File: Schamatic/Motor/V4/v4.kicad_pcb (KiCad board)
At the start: 4 copper layers, 40 x 25 mm, 45 parts, among them J1 SWD, J10 GND, J11 V, J12 U, J13 W, J2 SPI, J3 RS485, J4 RS485, J5 12, J6 12, J7 12, J8 GND, J9 GND, Q1 PSMN3R3-40YS, Q2 PSMN3R3-40YS, Q3 PSMN3R3-40YS, Q4 PSMN3R3-40YS, Q5 PSMN3R3-40YS, Q6 PSMN3R3-40YS, SW1 SWiTCH, SW2 SWiTCH, U1 STSPIN32F0, U2 RS-485, Y1 Resonator_Small

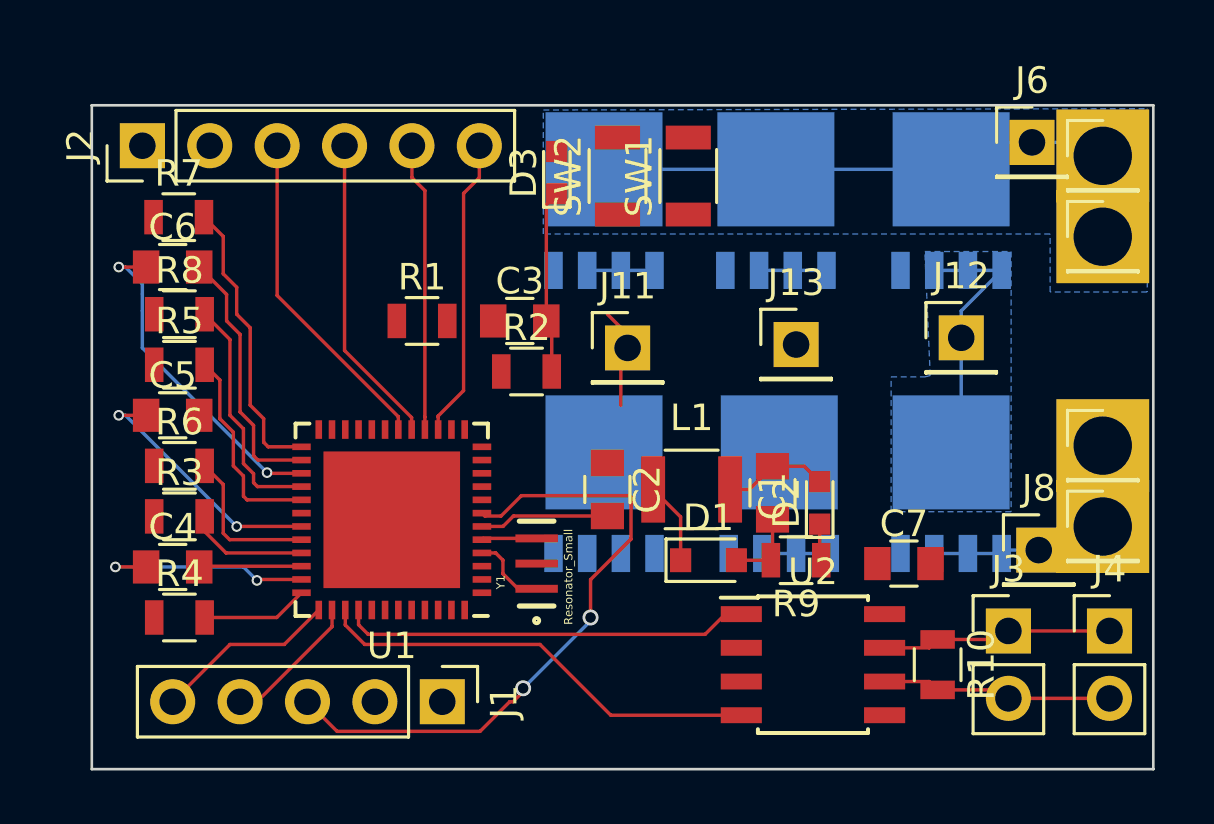
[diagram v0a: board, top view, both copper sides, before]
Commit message: ordered controller
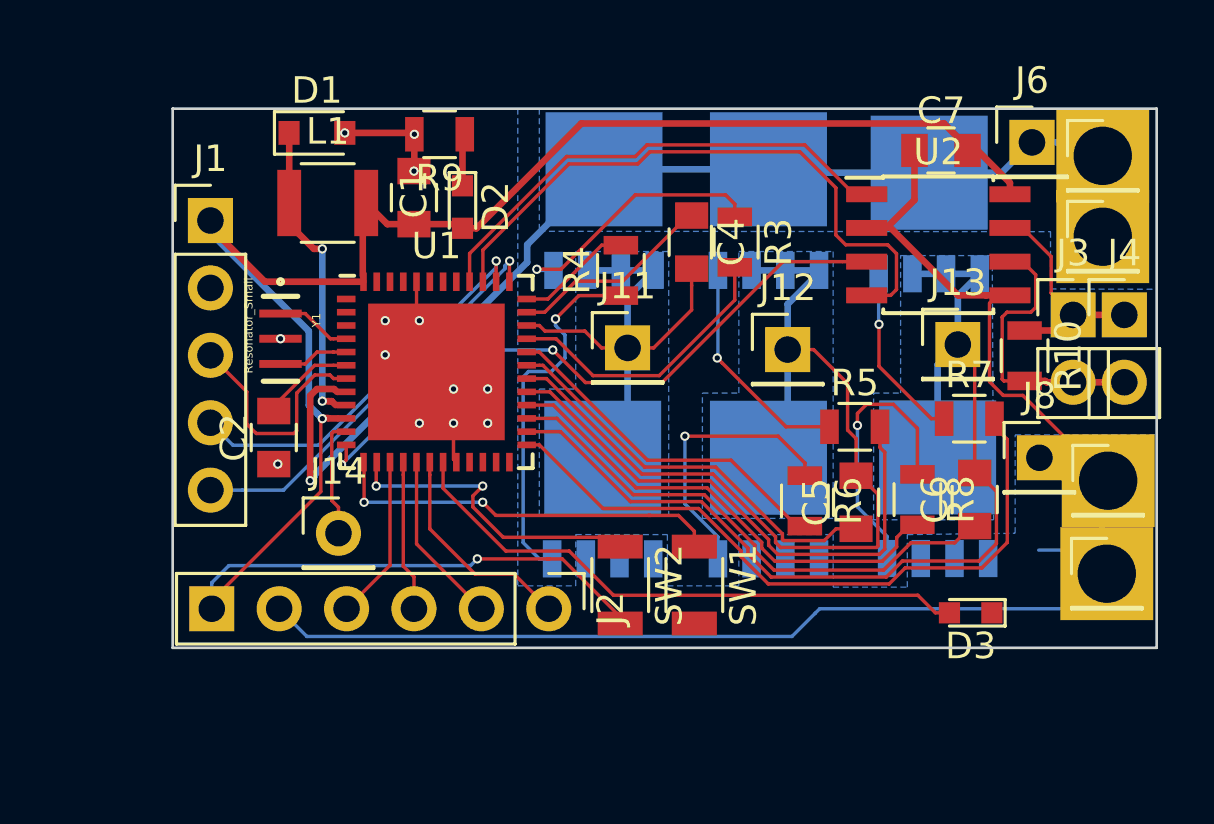
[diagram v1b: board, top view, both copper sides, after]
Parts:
- removed C3: 1uF, Capacitors_SMD:C_0805
- removed R1: 47K, Resistors_SMD:R_0805
- removed R2: 3K, Resistors_SMD:R_0805
- added J14: A0, Pin_Headers:Pin_Header_Straight_1x01_Pitch2.54mm, F.Cu at (109.4, 91.2)
- moved C6 31.5 mm to (133.3, 89.9), turned to 90 degrees
- moved R7 30.7 mm to (133.1, 86.9)
- moved R8 28.7 mm to (131.2, 89.9), turned to 270 degrees
- moved C5 26.0 mm to (128.9, 90.0), turned to 90 degrees
- moved R5 25.6 mm to (128.8, 87.2)
- moved R6 23.6 mm to (126.9, 90.0), turned to 270 degrees
- moved R3 23.3 mm to (124.3, 80.2), turned to 270 degrees
- moved J2 23.2 mm to (117.3, 94.0), turned to 270 degrees
- moved C4 23.1 mm to (122.7, 80.2), turned to 270 degrees
- moved D3 22.8 mm to (133.2, 94.2), turned to 180 degrees
- moved D1 21.8 mm to (108.6, 76.1)
- moved R4 21.2 mm to (120.0, 81.3), turned to 90 degrees
- moved R9 20.9 mm to (113.2, 76.1)
- moved J1 20.1 mm to (104.5, 79.4), turned to 0 degrees
- moved C1 17.5 mm to (112.2, 78.5), turned to 90 degrees
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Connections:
- J2 pad 1: +3V3 -> MOSI
- J2 pad 2: Earth -> MISO
- J2 pad 3: MOSI -> SCK
- J2 pad 4: MISO -> CS
- J2 pad 5: SCK -> Earth
- J2 pad 6: CS -> +3V3
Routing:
- net Earth: track 22.2 -> 93.2 mm, vias 0 -> 13
- net +3V3: track 3.98 -> 74.9 mm, vias 0 -> 2
- net O3: track 12.4 -> 39.3 mm
- net O2: track 10.2 -> 35.8 mm
- net DE: track 0.00 -> 24.8 mm, vias 0 -> 2
- net Net-(D3-Pad2): track 0.00 -> 22.0 mm
- net +12V: track 22.5 -> 44.4 mm, vias 0 -> 1
- net NRST: track 24.2 -> 8.86 mm, vias 2 -> 0
- net Net-(SW1-Pad1): track 0.00 -> 15.1 mm, vias 0 -> 2
- net H3: track 10.9 -> 25.9 mm
- net Net-(Q2-Pad4): track 0.00 -> 14.2 mm, vias 0 -> 1
- net H2: track 7.80 -> 20.9 mm
- net Net-(SW2-Pad1): track 0.00 -> 12.0 mm, vias 0 -> 2
- net Net-(Q4-Pad4): track 0.00 -> 10.6 mm, vias 0 -> 1
- net Net-(Q6-Pad4): track 0.00 -> 10.5 mm, vias 0 -> 1
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- added copper zone on B.Cu, net Earth
- added copper zone on B.Cu, net O1
- added copper zone on B.Cu, net O2
- added copper zone on B.Cu, net O3
- removed copper zone on B.Cu, net Net-(D3-Pad2)
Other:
- board size 40 x 25 mm -> 37.1 x 20.3 mm
- copper layers 4 -> 2
- net class Default: clearance 0.2 -> 0.13
- rule trace_clearance: 0.2 -> 0.13
- board text added: "3.3"
- board text added: "CS"
- board text added: "CSK"
- board text added: "GND"
- board text added: "MISO"
- board text added: "MOSI"
- board text added: "NRST"
- board text added: "SWDCLK"
- board text added: "SWDIO"
